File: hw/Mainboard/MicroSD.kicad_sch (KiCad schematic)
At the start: 6 parts, among them J24 MicroSD

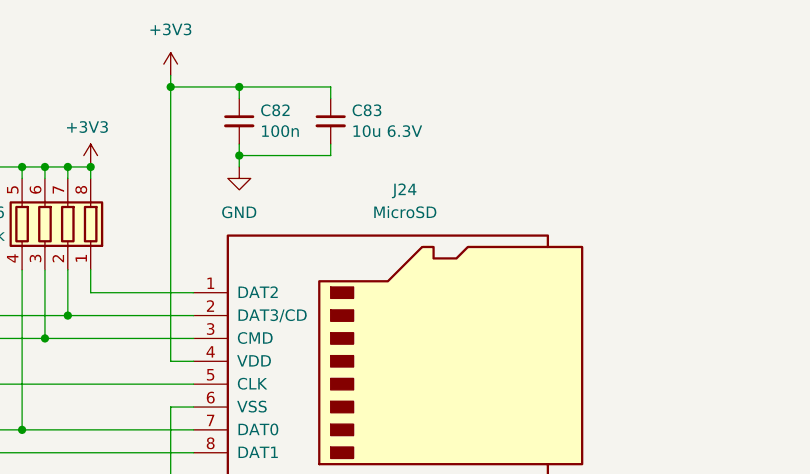
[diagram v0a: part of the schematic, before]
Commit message: hw: 25x2 header (wip)
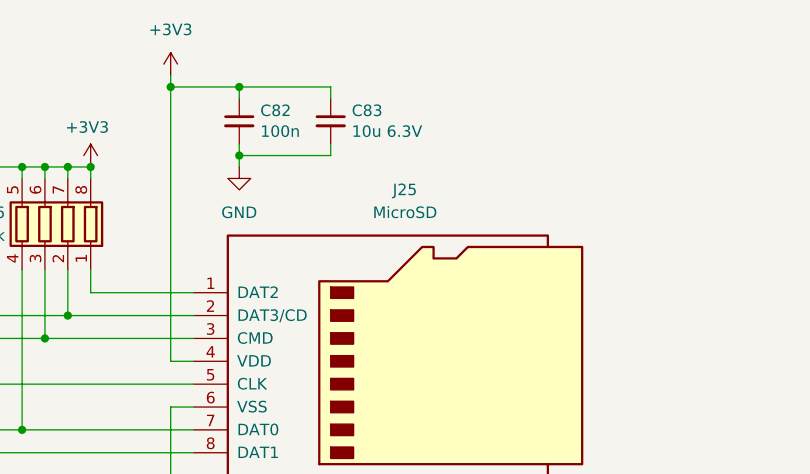
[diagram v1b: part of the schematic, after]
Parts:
- renumbered J24 to J25
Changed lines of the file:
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@@
   (symbol (lib_id "power:+3V3") (at 138.43 74.93 0) (mirror y) (unit 1)
     (in_bom yes) (on_board yes)
-    (property "Reference" "#PWR0145" (id 0) (at 138.43 78.74 0)
+    (property "Reference" "#PWR0147" (id 0) (at 138.43 78.74 0)
       (effects (font (size 1.27 1.27)) hide)
     )
@@
   (symbol (lib_id "power:+3V3") (at 147.32 64.77 0) (unit 1)
     (in_bom yes) (on_board yes)
-    (property "Reference" "#PWR0144" (id 0) (at 147.32 68.58 0)
+    (property "Reference" "#PWR0146" (id 0) (at 147.32 68.58 0)
       (effects (font (size 1.27 1.27)) hide)
     )
@@
   (symbol (lib_id "Connector:Micro_SD_Card_Det") (at 172.72 99.06 0) (unit 1)
     (in_bom yes) (on_board yes) (fields_autoplaced)
-    (property "Reference" "J24" (id 0) (at 173.355 77.47 0))
+    (property "Reference" "J25" (id 0) (at 173.355 77.47 0))
     (property "Value" "MicroSD" (id 1) (at 173.355 80.01 0))
     (property "Footprint" "JLCPCB:TF-SMD_TF-PUSH" (id 2) (at 224.79 81.28 0)
@@
   (symbol (lib_id "power:GND") (at 194.31 113.03 0) (unit 1)
     (in_bom yes) (on_board yes) (fields_autoplaced)
-    (property "Reference" "#PWR0147" (id 0) (at 194.31 119.38 0)
+    (property "Reference" "#PWR0149" (id 0) (at 194.31 119.38 0)
       (effects (font (size 1.27 1.27)) hide)
     )
@@
   (symbol (lib_id "power:GND") (at 147.32 118.11 0) (unit 1)
     (in_bom yes) (on_board yes) (fields_autoplaced)
-    (property "Reference" "#PWR0148" (id 0) (at 147.32 124.46 0)
+    (property "Reference" "#PWR0150" (id 0) (at 147.32 124.46 0)
       (effects (font (size 1.27 1.27)) hide)
     )
@@
   (symbol (lib_id "power:GND") (at 154.94 74.93 0) (unit 1)
     (in_bom yes) (on_board yes) (fields_autoplaced)
-    (property "Reference" "#PWR0146" (id 0) (at 154.94 81.28 0)
+    (property "Reference" "#PWR0148" (id 0) (at 154.94 81.28 0)
       (effects (font (size 1.27 1.27)) hide)
     )

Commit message: hw: 2x config switch (wip)
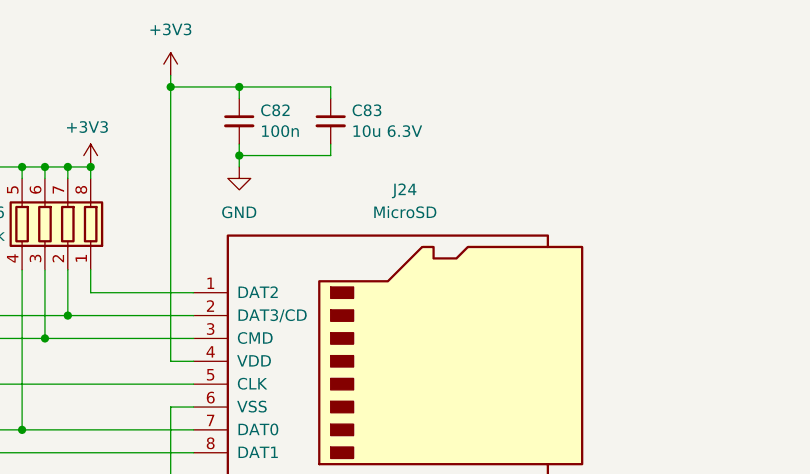
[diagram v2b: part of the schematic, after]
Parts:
- renumbered J25 to J24
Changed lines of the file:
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@@
   (symbol (lib_id "power:+3V3") (at 138.43 74.93 0) (mirror y) (unit 1)
     (in_bom yes) (on_board yes)
-    (property "Reference" "#PWR0147" (id 0) (at 138.43 78.74 0)
+    (property "Reference" "#PWR0153" (id 0) (at 138.43 78.74 0)
       (effects (font (size 1.27 1.27)) hide)
     )
@@
   (symbol (lib_id "power:+3V3") (at 147.32 64.77 0) (unit 1)
     (in_bom yes) (on_board yes)
-    (property "Reference" "#PWR0146" (id 0) (at 147.32 68.58 0)
+    (property "Reference" "#PWR0152" (id 0) (at 147.32 68.58 0)
       (effects (font (size 1.27 1.27)) hide)
     )
@@
   (symbol (lib_id "Connector:Micro_SD_Card_Det") (at 172.72 99.06 0) (unit 1)
     (in_bom yes) (on_board yes) (fields_autoplaced)
-    (property "Reference" "J25" (id 0) (at 173.355 77.47 0))
+    (property "Reference" "J24" (id 0) (at 173.355 77.47 0))
     (property "Value" "MicroSD" (id 1) (at 173.355 80.01 0))
     (property "Footprint" "JLCPCB:TF-SMD_TF-PUSH" (id 2) (at 224.79 81.28 0)
@@
   (symbol (lib_id "power:GND") (at 194.31 113.03 0) (unit 1)
     (in_bom yes) (on_board yes) (fields_autoplaced)
-    (property "Reference" "#PWR0149" (id 0) (at 194.31 119.38 0)
+    (property "Reference" "#PWR0155" (id 0) (at 194.31 119.38 0)
       (effects (font (size 1.27 1.27)) hide)
     )
@@
   (symbol (lib_id "power:GND") (at 147.32 118.11 0) (unit 1)
     (in_bom yes) (on_board yes) (fields_autoplaced)
-    (property "Reference" "#PWR0150" (id 0) (at 147.32 124.46 0)
+    (property "Reference" "#PWR0156" (id 0) (at 147.32 124.46 0)
       (effects (font (size 1.27 1.27)) hide)
     )
@@
   (symbol (lib_id "power:GND") (at 154.94 74.93 0) (unit 1)
     (in_bom yes) (on_board yes) (fields_autoplaced)
-    (property "Reference" "#PWR0148" (id 0) (at 154.94 81.28 0)
+    (property "Reference" "#PWR0154" (id 0) (at 154.94 81.28 0)
       (effects (font (size 1.27 1.27)) hide)
     )
